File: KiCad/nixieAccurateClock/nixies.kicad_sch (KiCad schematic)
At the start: 6 parts

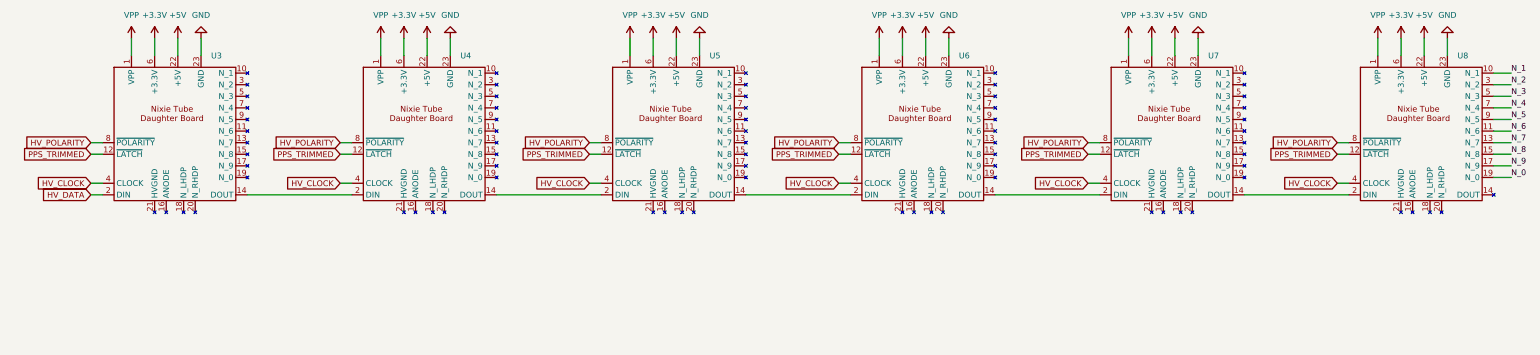
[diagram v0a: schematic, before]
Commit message: simplify nixie daughter board
Remove cathode pins that would not be usable for current sensing anyway.
Pivot to using anode pin as shunt measurement with a R2R flash ADC (not yet implemented).
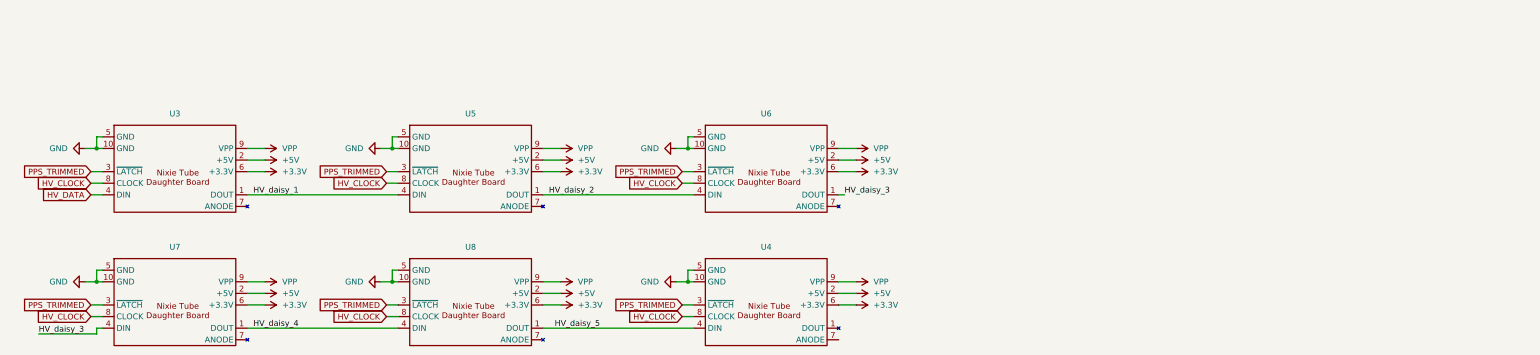
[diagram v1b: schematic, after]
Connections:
- net HV_POLARITY is gone; now on net HV_CLOCK: U3.8 (CLOCK), U4.8 (CLOCK), U5.8 (CLOCK), U6.8 (CLOCK), U7.8 (CLOCK), U8.8 (CLOCK)
- net N_1 is gone; now on net GND: U8.10 (GND)
- net N_2 is gone; now on net PPS_TRIMMED: U8.3 (~{LATCH})
- net N_3 is gone; now on net GND: U8.5 (GND)
- net N_5 is gone; now on net VPP: U8.9 (VPP)
- net +5V: now also U3.2 (+5V), U4.2 (+5V), U5.2 (+5V), U6.2 (+5V), U7.2 (+5V), U8.2 (+5V); no longer U3.22 (+5V), U4.22 (+5V), U5.22 (+5V), U6.22 (+5V), U7.22 (+5V), U8.22 (+5V)
- net GND: now also U3.10 (GND), U3.5 (GND), U4.10 (GND), U4.5 (GND), U5.10 (GND), U5.5 (GND), U6.10 (GND), U6.5 (GND), U7.10 (GND), U7.5 (GND); no longer U3.23 (GND), U4.23 (GND), U5.23 (GND), U6.23 (GND), U7.23 (GND), U8.23 (GND)
- net HV_CLOCK: no longer U3.4 (CLOCK), U4.4 (CLOCK), U5.4 (CLOCK), U6.4 (CLOCK), U7.4 (CLOCK), U8.4 (CLOCK)
- net HV_DATA: now also U3.4 (DIN); no longer U3.2 (DIN)
- net PPS_TRIMMED: now also U3.3 (~{LATCH}), U4.3 (~{LATCH}), U5.3 (~{LATCH}), U6.3 (~{LATCH}), U7.3 (~{LATCH}); no longer U3.12 (~{LATCH}), U4.12 (~{LATCH}), U5.12 (~{LATCH}), U6.12 (~{LATCH}), U7.12 (~{LATCH}), U8.12 (~{LATCH})
- net VPP: now also U3.9 (VPP), U4.9 (VPP), U5.9 (VPP), U6.9 (VPP), U7.9 (VPP); no longer U3.1 (VPP), U4.1 (VPP), U5.1 (VPP), U6.1 (VPP), U7.1 (VPP), U8.1 (VPP)
- removed net N_0: U8.19 (N_0)
- net N_4: no longer names the net of U8.7 (ANODE)
- removed net N_6: U8.11 (N_6)
- removed net N_7: U8.13 (N_7)
- removed net N_8: U8.15 (N_8)
- removed net N_9: U8.17 (N_9)
- new net HV_daisy_1: U3.1 (DOUT), U5.4 (DIN)
- new net HV_daisy_2: U5.1 (DOUT), U6.4 (DIN)
- new net HV_daisy_3: U6.1 (DOUT), U7.4 (DIN)
- new net HV_daisy_4: U7.1 (DOUT), U8.4 (DIN)
- new net HV_daisy_5: U4.4 (DIN), U8.1 (DOUT)
